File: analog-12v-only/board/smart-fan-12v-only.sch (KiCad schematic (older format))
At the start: 34 parts, among them J1 TEMP_In, J2 12V_PWR, J3 12V_In, J4 FAN_Out, J5 FAN_Out, J6 FAN_Out, Q1 BC817, Q2 Q_PMOS_GSD, Q3 Q_PMOS_GSD, Q4 BC817, U1 MCP602, U2 AMS1117-5.0, U3 NE555P

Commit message: Board layout complete with ground planes and mounting holes
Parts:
- removed C3: 1uF, Resistor_SMD:R_0805_2012Metric_Pad1.15x1.40mm_HandSolder, symbol Device:CP
- removed J1: TEMP_In, Connector_PinHeader_1.27mm:PinHeader_1x03_P1.27mm_Vertical, symbol smart-fan-rescue:Conn_01x03_MountingPin-ConnectorMountingPin
- removed J6: FAN_Out, Connector:FanPinHeader_1x03_P2.54mm_Vertical, symbol Connector:Conn_01x03_Male
- removed Q1, Q4: BC817, Package_TO_SOT_SMD:SOT-23, symbol smart-fan-rescue:BC817-TransistorBJT
- removed Q2: Q_PMOS_GSD, Package_TO_SOT_SMD:TO-263-2, symbol Device:Q_PMOS_GSD
- removed Q3: Q_PMOS_GSD, Package_TO_SOT_SMD:SOT-23, symbol Device:Q_PMOS_GSD
- removed R11: 560, Resistor_SMD:R_0805_2012Metric_Pad1.15x1.40mm_HandSolder, symbol Device:R
- removed U2: AMS1117-5.0, Package_TO_SOT_SMD:SOT-223-3_TabPin2, symbol smart-fan-rescue:AMS1117-5.0-Reg_Linear
- added D3: GREEN_LED, LED_THT:LED_D3.0mm, symbol Device:LED_Small
- added J1: KTY81/120, Connector_Pin254mm:PinSocket_1x02_P2.54mm_Vertical, symbol ConnectorMountingPin:Conn_01x02_MountingPin
- added Q1: 2N3904, Package_TO_SOT_THT:TO-92_Inline, symbol TransistorBJT:2N3904
- added Q2: FQP27P06, Package_TO_SOT_THT:TO-220-3_Vertical, symbol TransistorFET:FQP27P06
- added R12: 27k, Resistor_THT:R_Axial_DIN0204_L3.6mm_D1.6mm_P2.54mm_Vertical, symbol Device:R
- C1: value 1uF -> 10uF; footprint Resistor_SMD:R_0805_2012Metric_Pad1.15x1.40mm_HandSolder -> Capacitor_THT:CP_Radial_D5.0mm_P2.00mm
- C2, C4, C5, C7: footprint Resistor_SMD:R_0805_2012Metric_Pad1.15x1.40mm_HandSolder -> Capacitor_THT:C_Rect_L4.0mm_W2.5mm_P2.50mm
- C6: footprint Capacitor_SMD:C_1812_4532Metric_Pad1.30x3.40mm_HandSolder -> Capacitor_THT:CP_Radial_D7.5mm_P2.50mm
- D1: footprint Resistor_SMD:R_0805_2012Metric_Pad1.15x1.40mm_HandSolder -> LED_THT:LED_D3.0mm
- D2: footprint Diode_SMD:D_1210_3225Metric_Pad1.42x2.65mm_HandSolder -> Diode_THT:D_A-405_P2.54mm_Vertical_AnodeUp
- J2: footprint Connector_BarrelJack:BarrelJack_CUI_PJ-063AH_Horizontal_CircularHoles -> Connector_BarrelJack:BarrelJack_Horizontal
- R1, R2, R3, R4, R5, R6, R7, R8, R9: footprint Resistor_SMD:R_0805_2012Metric_Pad1.15x1.40mm_HandSolder -> Resistor_THT:R_Axial_DIN0204_L3.6mm_D1.6mm_P2.54mm_Vertical
- R10: value 6.8k -> 10k; footprint Resistor_SMD:R_0805_2012Metric_Pad1.15x1.40mm_HandSolder -> Resistor_THT:R_Axial_DIN0204_L3.6mm_D1.6mm_P2.54mm_Vertical
- RV1: value 10k -> 100k
- U1: value MCP602 -> LM358; footprint Package_SO:SOIC-8_5.275x5.275mm_P1.27mm -> Package_DIP:DIP-8_W7.62mm_Socket
- U3: footprint Package_SO:SOIC-8_5.275x5.275mm_P1.27mm -> Package_DIP:DIP-8_W7.62mm_Socket
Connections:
- net labels removed: +5V
- wire segments 140 -> 121
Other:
- moved on the sheet: J2, J3, RV1

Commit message: Fix up 12v only analog fan controller
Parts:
- J1: symbol ConnectorMountingPin:Conn_01x02_MountingPin -> smart-fan-12v-only-rescue:Conn_01x02_MountingPin-ConnectorMountingPin
- Q1: symbol TransistorBJT:2N3904 -> smart-fan-12v-only-rescue:2N3904-TransistorBJT
- Q2: symbol TransistorFET:FQP27P06 -> smart-fan-12v-only-rescue:FQP27P06-TransistorFET
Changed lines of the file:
@@
 EELAYER 30 0
 EELAYER END
-$Descr A0 46811 33110
+$Descr A4 11693 8268
 encoding utf-8
 Sheet 1 1
@@
 	6300 4900 6300 5400
 $Comp
-L TransistorBJT:2N3904 Q1
+L smart-fan-12v-only-rescue:2N3904-TransistorBJT Q1
 U 1 1 5EF082D2
 P 4800 4650
@@
 $EndComp
 $Comp
-L TransistorFET:FQP27P06 Q2
+L smart-fan-12v-only-rescue:FQP27P06-TransistorFET Q2
 U 1 1 5EF09F99
 P 5500 4250
@@
 	5650 2350 6400 2350
 $Comp
-L ConnectorMountingPin:Conn_01x02_MountingPin J1
+L smart-fan-12v-only-rescue:Conn_01x02_MountingPin-ConnectorMountingPin J1
 U 1 1 5EF516C3
 P 2100 2450

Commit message: Layout fixes and stable power
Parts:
- removed Q1: 2N3904, Package_TO_SOT_THT:TO-92_Inline, symbol smart-fan-12v-only-rescue:2N3904-TransistorBJT
- removed R6: 2.2k, Resistor_THT:R_Axial_DIN0204_L3.6mm_D1.6mm_P2.54mm_Vertical, symbol Device:R
- added C3: 10uF, Capacitor_THT:CP_Radial_D5.0mm_P2.00mm, symbol Device:CP
- added Q1: 2N7000, Package_TO_SOT_THT:TO-92_Inline, symbol TransistorFET:2N7000
- added U2: L7809, Package_TO_SOT_THT:TO-92, symbol Reg_Linear:L7809
- D2: value D_Schottky -> 1N5818
- R1: value 1M -> 100k
- R2: value 9.2k -> 1k5
- R3: value 82k -> 3k
- R4: value 100k -> 1M
- R5: value 2.2k -> 1k
- R7: value 2.2k -> 100k
- R8: value 68k -> 10k
- RV1: value 100k -> 10k
- U1: symbol smart-fan-rescue:MCP602-AmpOperational -> smart-fan-12v-only-rescue:MCP602-AmpOperational-smart-fan-rescue
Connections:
- net labels added: +9V
- wire segments 121 -> 129

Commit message: Fix board layout
Power transistor drain-source swapped
Flyback diode reversed
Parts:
- C6: value 100uF -> 330uF
- D2: value 1N5818 -> 1N5820
- J3: footprint Connector_PinSocket_2.54mm:PinSocket_1x02_P2.54mm_Vertical -> TerminalBlock_Phoenix:TerminalBlock_Phoenix_MKDS-1,5-2_1x02_P5.00mm_Horizontal
- Q1: symbol TransistorFET:2N7000 -> smart-fan-12v-only-rescue:2N7000-TransistorFET
- R12: value 27k -> 5k
- R9: value 27k -> 3k3
- U2: symbol Reg_Linear:L7809 -> smart-fan-12v-only-rescue:L7809-Reg_Linear
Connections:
- wire segments 129 -> 130
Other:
- moved on the sheet: D1, R9
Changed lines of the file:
@@
 L Device:R R9
 U 1 1 5EE89D31
-P 5600 4750
-F 0 "R9" H 5670 4796 50  0000 L CNN
-F 1 "27k" H 5670 4705 50  0000 L CNN
-F 2 "Resistor_THT:R_Axial_DIN0204_L3.6mm_D1.6mm_P2.54mm_Vertical" V 5530 4750 50  0001 C CNN
-F 3 "~" H 5600 4750 50  0001 C CNN
-	1    5600 4750
+P 4250 4950
+F 0 "R9" H 4320 4996 50  0000 L CNN
+F 1 "3k3" H 4320 4905 50  0000 L CNN
+F 2 "Resistor_THT:R_Axial_DIN0204_L3.6mm_D1.6mm_P2.54mm_Vertical" V 4180 4950 50  0001 C CNN
+F 3 "~" H 4250 4950 50  0001 C CNN
+	1    4250 4950
 	1    0    0    -1
 $EndComp
@@
 L Device:LED_Small D1
 U 1 1 5EE8AC2E
-P 5600 5100
-F 0 "D1" V 5646 5030 50  0000 R CNN
-F 1 "RED_LED" V 5555 5030 50  0000 R CNN
-F 2 "LED_THT:LED_D3.0mm" V 5600 5100 50  0001 C CNN
-F 3 "~" V 5600 5100 50  0001 C CNN
-	1    5600 5100
+P 4250 5300
+F 0 "D1" V 4296 5230 50  0000 R CNN
+F 1 "RED_LED" V 4205 5230 50  0000 R CNN
+F 2 "LED_THT:LED_D3.0mm" V 4250 5300 50  0001 C CNN
+F 3 "~" V 4250 5300 50  0001 C CNN
+	1    4250 5300
 	0    -1   -1   0
 $EndComp
@@
 	4900 5400 5250 5400
 Wire Wire Line
-	5600 5400 5600 5200
-Wire Wire Line
-	5600 4600 5600 4550
+	4250 5600 4250 5400
 Wire Wire Line
 	5600 4550 6000 4550
@@
 P 3650 5350
 F 0 "C6" H 3768 5396 50  0000 L CNN
-F 1 "100uF" H 3768 5305 50  0000 L CNN
+F 1 "330uF" H 3768 5305 50  0000 L CNN
 F 2 "Capacitor_THT:CP_Radial_D7.5mm_P2.50mm" H 3688 5200 50  0001 C CNN
 F 3 "~" H 3650 5350 50  0001 C CNN
@@
 F 0 "J3" H 3230 1042 50  0000 L CNN
 F 1 "12V_In" H 3230 951 50  0000 L CNN
-F 2 "Connector_PinSocket_2.54mm:PinSocket_1x02_P2.54mm_Vertical" H 3150 1050 50  0001 C CNN
+F 2 "TerminalBlock_Phoenix:TerminalBlock_Phoenix_MKDS-1,5-2_1x02_P5.00mm_Horizontal" H 3150 1050 50  0001 C CNN
 F 3 "~" H 3150 1050 50  0001 C CNN
 	1    3150 1050
@@
 Trigger
 Wire Wire Line
-	5600 4900 5600 5000
+	4250 5100 4250 5200
 $Comp
 L Connector:Conn_01x03_Male J5
@@
 P 5250 4900
 F 0 "D2" V 5296 4820 50  0000 R CNN
-F 1 "1N5818" V 5205 4820 50  0000 R CNN
+F 1 "1N5820" V 5205 4820 50  0000 R CNN
 F 2 "Diode_THT:D_A-405_P2.54mm_Vertical_AnodeUp" H 5250 4900 50  0001 C CNN
 F 3 "~" H 5250 4900 50  0001 C CNN
 	1    5250 4900
-	0    -1   -1   0
+	0    1    1    0
 $EndComp
 Wire Wire Line
@@
 F 3 "https://www.onsemi.com/pub/Collateral/FQP27P06-D.PDF" H 5500 4250 50  0001 L CNN
 	1    5500 4250
-	1    0    0    -1
+	1    0    0    1
 $EndComp
 $Comp
@@
 P 1250 1150
 F 0 "R12" H 1320 1196 50  0000 L CNN
-F 1 "27k" H 1320 1105 50  0000 L CNN
+F 1 "5k" H 1320 1105 50  0000 L CNN
 F 2 "Resistor_THT:R_Axial_DIN0204_L3.6mm_D1.6mm_P2.54mm_Vertical" V 1180 1150 50  0001 C CNN
 F 3 "~" H 1250 1150 50  0001 C CNN
@@
 	2700 2150 2700 2350
 $Comp
-L TransistorFET:2N7000 Q1
+L smart-fan-12v-only-rescue:2N7000-TransistorFET Q1
 U 1 1 5EEC101F
 P 4800 4650
@@
 $EndComp
 $Comp
-L Reg_Linear:L7809 U2
+L smart-fan-12v-only-rescue:L7809-Reg_Linear U2
 U 1 1 5EEC3711
 P 7100 1000
@@
 $EndComp
 $Comp
-L Power:+9V #PWR0102
+L smart-fan-12v-only-rescue:+9V-Power #PWR0102
 U 1 1 5EED8706
 P 7650 800
@@
 	6650 1000 6650 800
 $Comp
-L Power:+9V #PWR0104
+L smart-fan-12v-only-rescue:+9V-Power #PWR0104
 U 1 1 5EEE3C6D
 P 4300 1300
@@
 $EndComp
 $Comp
-L Power:+9V #PWR0105
+L smart-fan-12v-only-rescue:+9V-Power #PWR0105
 U 1 1 5EEE4039
 P 2700 1700
@@
 $EndComp
 $Comp
-L Power:+9V #PWR0110
+L smart-fan-12v-only-rescue:+9V-Power #PWR0110
 U 1 1 5EEE44AD
 P 3000 3950
@@
 $EndComp
 $Comp
-L Power:+9V #PWR0117
+L smart-fan-12v-only-rescue:+9V-Power #PWR0117
 U 1 1 5EEE4AEF
 P 1150 2750
@@
 $EndComp
 Wire Wire Line
-	3500 4650 4600 4650
+	3500 4650 4250 4650
+Wire Wire Line
+	4250 4650 4250 4800
+Connection ~ 4250 4650
+Wire Wire Line
+	4250 4650 4600 4650
+$Comp
+L smart-fan-12v-only-rescue:GND-Power-smart-fan-rescue #PWR0118
+U 1 1 5F016451
+P 4250 5600
+F 0 "#PWR0118" H 4250 5350 50  0001 C CNN
+F 1 "GND" H 4255 5427 50  0000 C CNN
+F 2 "" H 4250 5600 50  0001 C CNN
+F 3 "" H 4250 5600 50  0001 C CNN
+	1    4250 5600
+	1    0    0    -1
+$EndComp
 $EndSCHEMATC

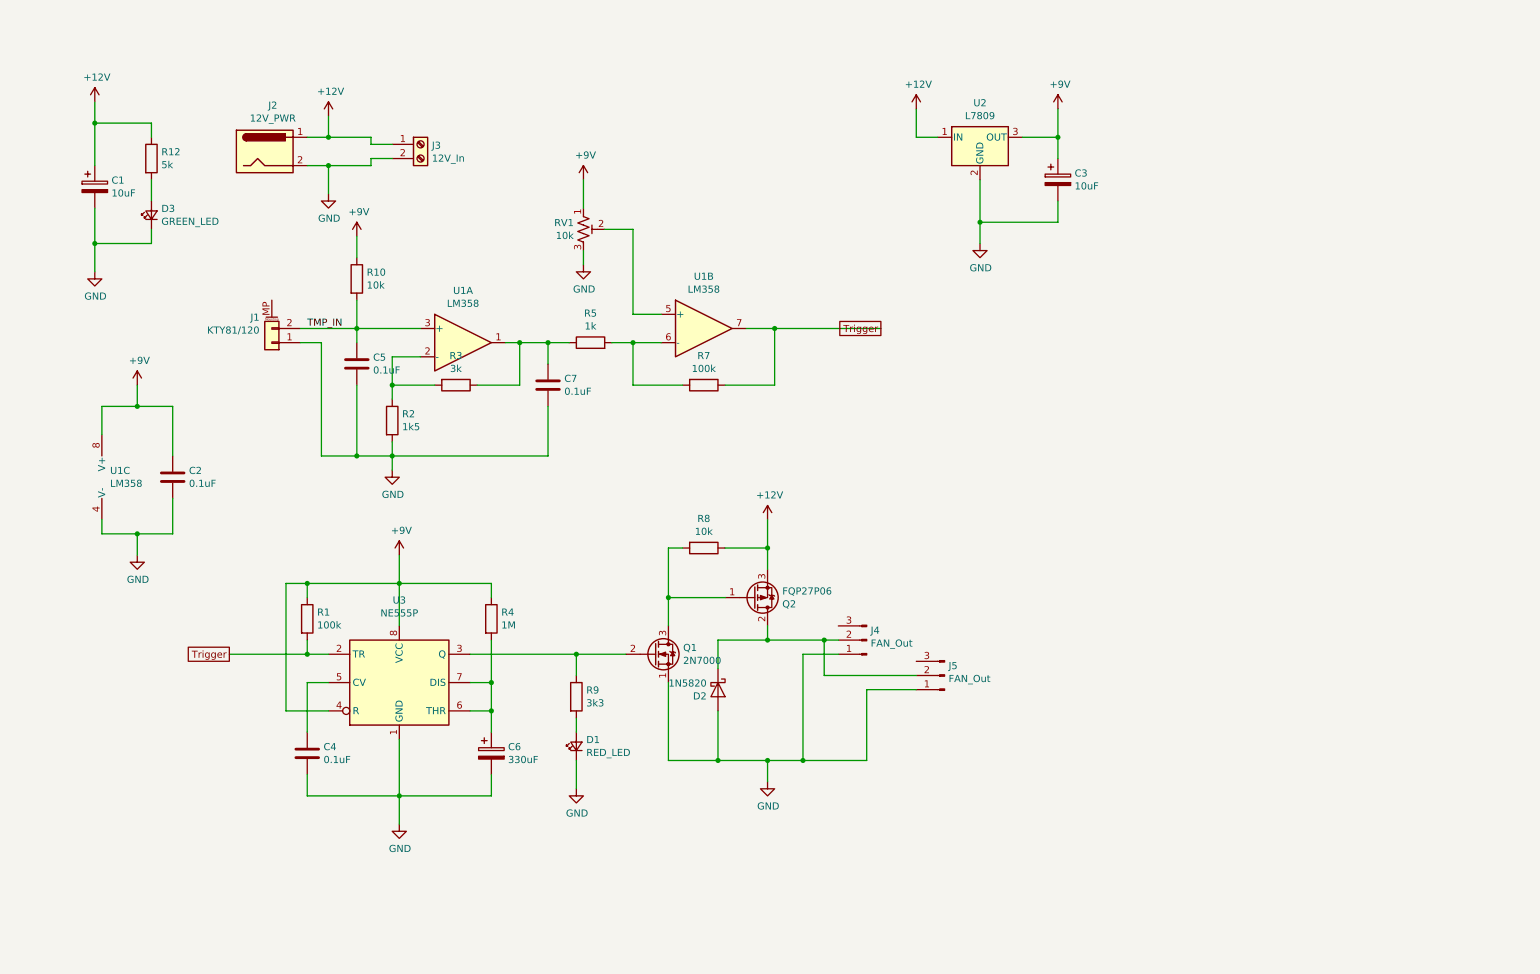
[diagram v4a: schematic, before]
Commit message: WIP: Cleaning up board
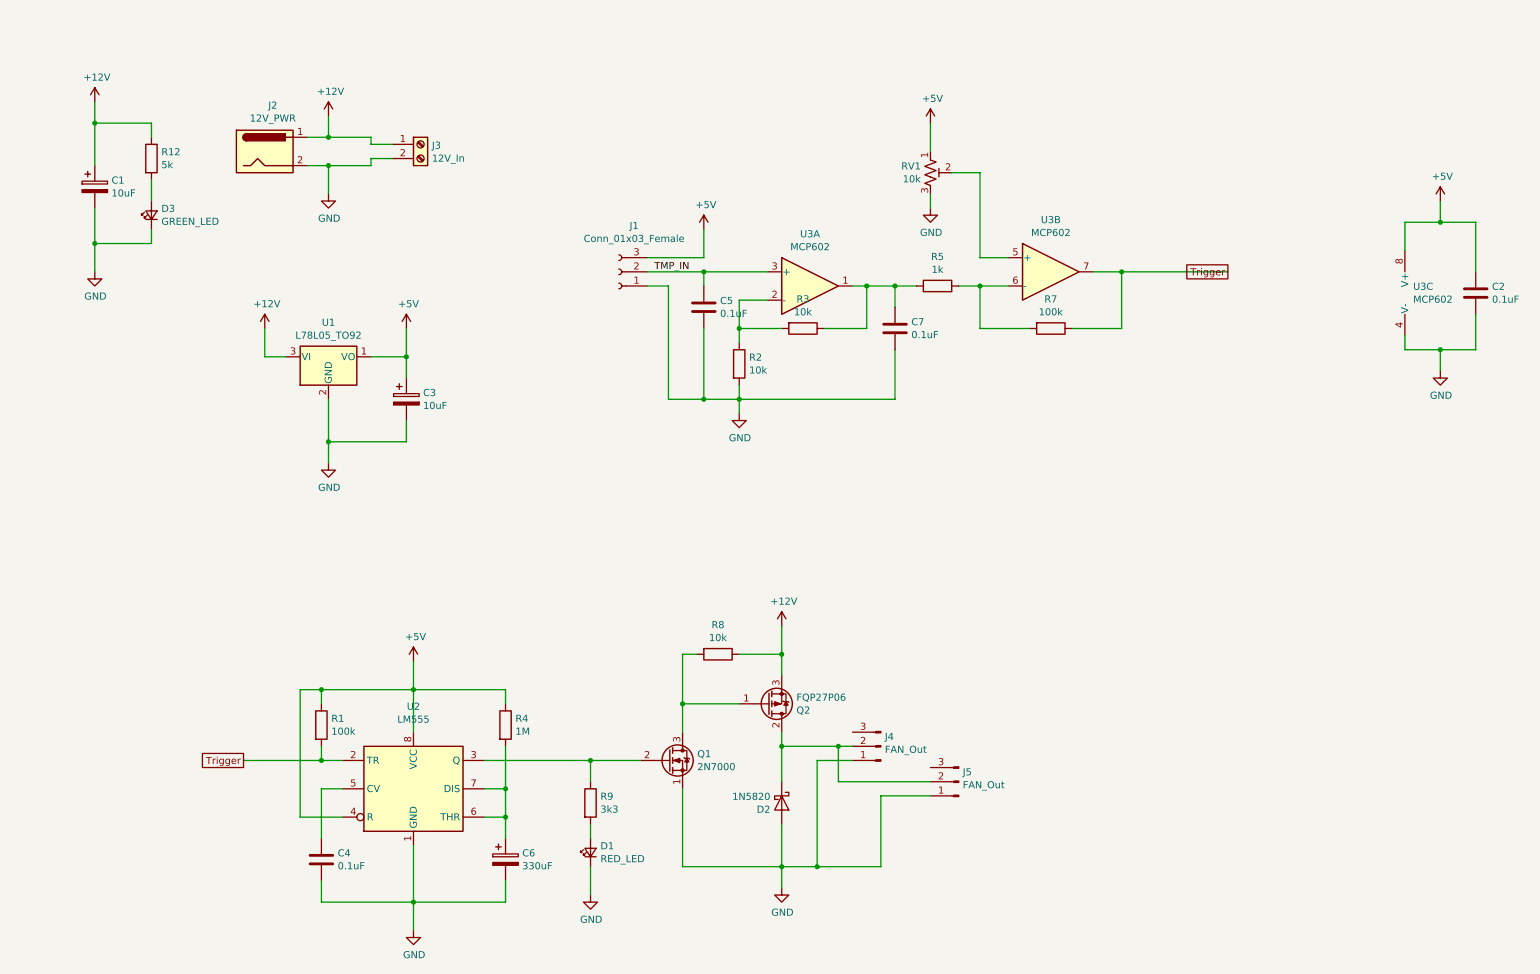
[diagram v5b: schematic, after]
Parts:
- removed J1: KTY81/120, Connector_Pin254mm:PinSocket_1x02_P2.54mm_Vertical, symbol smart-fan-12v-only-rescue:Conn_01x02_MountingPin-ConnectorMountingPin
- removed R10: 10k, Resistor_THT:R_Axial_DIN0204_L3.6mm_D1.6mm_P2.54mm_Vertical, symbol Device:R
- removed U1: LM358, Package_DIP:DIP-8_W7.62mm_Socket, symbol smart-fan-12v-only-rescue:MCP602-AmpOperational-smart-fan-rescue
- removed U2: L7809, Package_TO_SOT_THT:TO-92, symbol smart-fan-12v-only-rescue:L7809-Reg_Linear
- removed U3: NE555P, Package_DIP:DIP-8_W7.62mm_Socket, symbol Timer:NE555P
- added J1: Conn_01x03_Female, Connector_PinSocket_2.54mm:PinSocket_1x03_P2.54mm_Vertical, symbol Connector:Conn_01x03_Female
- added U1: L78L05_TO92, Package_TO_SOT_THT:TO-92_Inline, symbol Regulator_Linear:L78L05_TO92
- added U2: LM555, Package_DIP:DIP-8_W7.62mm_Socket, symbol Timer:LM555
- added U3: MCP602, Package_DIP:DIP-8_W7.62mm_Socket, symbol Amplifier_Operational:MCP602
- Q2: footprint Package_TO_SOT_THT:TO-220-3_Vertical -> Package_TO_SOT_THT:TO-251-3-1EP_Horizontal_TabDown
- R2: value 1k5 -> 10k
- R3: value 3k -> 10k
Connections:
- net +12V: now also U1.3 (VI)
- net GND: now also J1.1 (Pin_1), U1.2 (GND), U2.1 (GND), U3.4 (V-)
- net TMP_IN: now also J1.2 (Pin_2), U3.3 (+)
- net Trigger: now also U2.2 (TR), U3.7
- net at C7.1, R3.1, R5.1: now also U3.1
- net at R5.2, R7.2: now also U3.6 (-)
- net at R2.1, R3.2: now also U3.2 (-)
- net at RV1.2: now also U3.5 (+)
- net at Q1.2 (G), R9.1: now also U2.3 (Q)
- net at C4.1: now also U2.5 (CV)
- net at C6.1, R4.2: now also U2.6 (THR), U2.7 (DIS)
- net +9V renamed +5V
- net +5V: now also J1.3 (Pin_3), U1.1 (VO), U2.4 (R), U2.8 (VCC), U3.8 (V+)
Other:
- moved on the sheet: C2, C3, C4, C5, C6, C7, D1, D2, J4, J5, Q1, Q2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
